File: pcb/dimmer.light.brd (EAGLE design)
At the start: 45.7 x 45.4 mm, 25 parts, among them IC1 NCP1117ST50T3G, SW1 RJ45SMD, T1 IRFR024NPBF, T2 BC847BSMD, U1 ATTINY2313

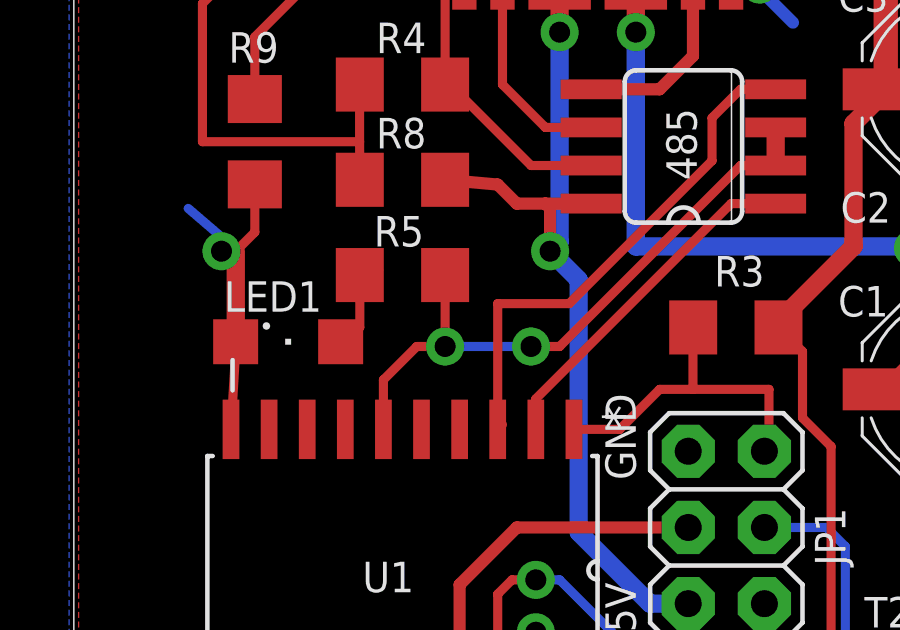
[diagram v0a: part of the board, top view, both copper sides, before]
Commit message: final version
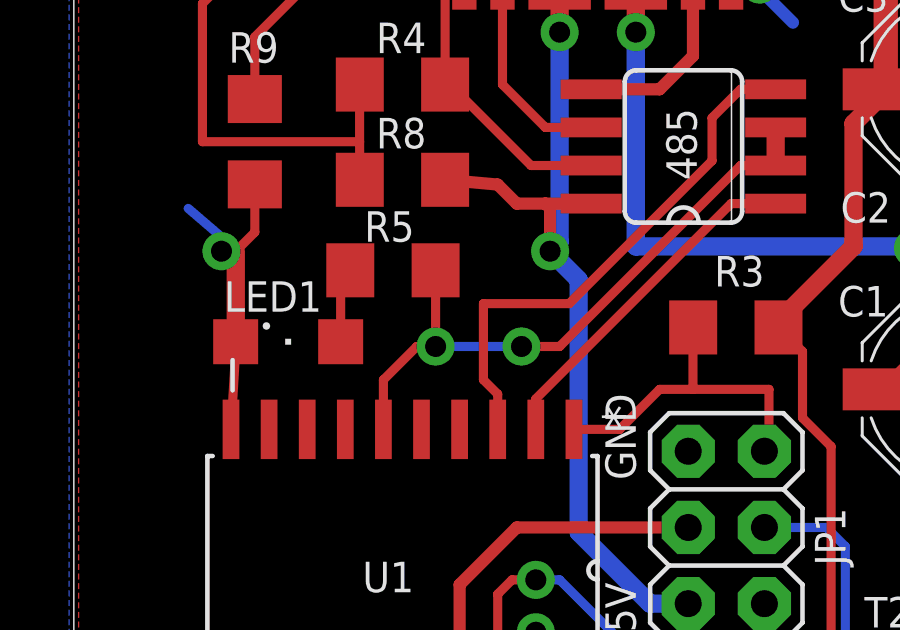
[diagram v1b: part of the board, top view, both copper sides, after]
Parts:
- R4: value 120 -> 220
- moved R5 0.35 mm to (12.9, 24.8)
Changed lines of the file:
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@@
 <attribute name="NAME" x="21.971" y="30.1625" size="1.016" layer="25" ratio="10" rot="R270"/>
 </element>
-<element name="R4" library="rcl" package="R1206" value="120" x="13.17625" y="30.95625" smashed="yes" rot="R180">
+<element name="R4" library="rcl" package="R1206" value="220" x="13.17625" y="30.95625" smashed="yes" rot="R180">
 <attribute name="NAME" x="13.97" y="33.02" size="1.016" layer="25" rot="R180"/>
 <attribute name="VALUE" x="14.44625" y="33.49625" size="1.27" layer="27" rot="R180"/>
@@
 <attribute name="VALUE" x="7.86625" y="19.88375" size="1.27" layer="27"/>
 </element>
-<element name="R5" library="rcl" package="R1206" value="680" x="13.17625" y="24.60625" smashed="yes">
-<attribute name="NAME" x="12.22375" y="25.55875" size="1.016" layer="25"/>
-<attribute name="VALUE" x="11.90625" y="22.06625" size="1.27" layer="27"/>
+<element name="R5" library="rcl" package="R1206" value="680" x="12.85875" y="24.765" smashed="yes">
+<attribute name="NAME" x="11.90625" y="25.7175" size="1.016" layer="25"/>
+<attribute name="VALUE" x="11.58875" y="22.225" size="1.27" layer="27"/>
 </element>
 <element name="R8" library="rcl" package="R1206" value="10k" x="13.17625" y="27.78125" smashed="yes">
@@
 <contactref element="LED1" pad="A"/>
 <contactref element="R5" pad="1"/>
-<wire x1="12.3855" y1="24.76875" x2="11.75425" y2="24.60625" width="0.3048" layer="1"/>
-<wire x1="11.75425" y1="24.60625" x2="11.75425" y2="22.863" width="0.3048" layer="1"/>
-<wire x1="11.75425" y1="22.863" x2="11.11625" y2="22.38375" width="0.3048" layer="1"/>
+<wire x1="11.43675" y1="24.765" x2="11.11625" y2="24.765" width="0.3048" layer="1"/>
+<wire x1="11.11625" y1="24.765" x2="11.11625" y2="22.38375" width="0.3048" layer="1"/>
 </signal>
 <signal name="N$18">
 <contactref element="485" pad="4"/>
 <contactref element="U1" pad="3"/>
-<wire x1="16.51" y1="19.6215" x2="16.35125" y2="19.46275" width="0.3048" layer="1"/>
 <wire x1="23.495" y1="28.41625" x2="18.7325" y2="23.65375" width="0.3048" layer="1"/>
-<wire x1="18.7325" y1="23.65375" x2="16.35125" y2="23.65375" width="0.3048" layer="1"/>
-<wire x1="16.35125" y1="23.65375" x2="16.35125" y2="19.46275" width="0.3048" layer="1"/>
+<wire x1="18.7325" y1="23.65375" x2="15.875" y2="23.65375" width="0.3048" layer="1"/>
 <wire x1="23.495" y1="28.41625" x2="23.495" y2="29.845" width="0.3048" layer="1"/>
 <wire x1="23.495" y1="29.845" x2="24.4475" y2="30.7975" width="0.3048" layer="1"/>
 <wire x1="24.4475" y1="30.7975" x2="25.6159" y2="30.7975" width="0.3048" layer="1"/>
+<wire x1="15.875" y1="23.65375" x2="15.875" y2="21.11375" width="0.3048" layer="1"/>
+<wire x1="15.875" y1="21.11375" x2="16.35125" y2="20.6375" width="0.3048" layer="1"/>
+<wire x1="16.35125" y1="20.6375" x2="16.35125" y2="19.46275" width="0.3048" layer="1"/>
 </signal>
 <signal name="N$19">
@@
 <contactref element="U1" pad="6"/>
 <wire x1="24.4475" y1="28.2575" x2="25.6159" y2="28.2575" width="0.3048" layer="1"/>
-<via x="17.4625" y="22.225" extent="1-16" drill="0.7" diameter="1.27" shape="square"/>
-<wire x1="14.605" y1="22.225" x2="14.59825" y2="22.225" width="0.3048" layer="16"/>
+<via x="17.145" y="22.225" extent="1-16" drill="0.7" diameter="1.27" shape="square"/>
+<wire x1="14.605" y1="22.225" x2="14.28075" y2="22.225" width="0.3048" layer="16"/>
 <wire x1="12.54125" y1="19.46275" x2="12.54125" y2="21.11375" width="0.3048" layer="1"/>
 <wire x1="12.54125" y1="21.11375" x2="13.6525" y2="22.225" width="0.3048" layer="1"/>
-<wire x1="13.6525" y1="22.225" x2="14.59825" y2="22.225" width="0.3048" layer="1"/>
-<via x="14.59825" y="22.225" extent="1-16" drill="0.7" diameter="1.27" shape="square"/>
-<wire x1="14.59825" y1="22.225" x2="17.4625" y2="22.225" width="0.3048" layer="16"/>
-<wire x1="14.59825" y1="24.60625" x2="14.59825" y2="22.225" width="0.3048" layer="1"/>
-<wire x1="17.4625" y1="22.225" x2="18.415" y2="22.225" width="0.3048" layer="1"/>
+<wire x1="13.6525" y1="22.225" x2="14.28075" y2="22.225" width="0.3048" layer="1"/>
+<via x="14.28075" y="22.225" extent="1-16" drill="0.7" diameter="1.27" shape="square"/>
+<wire x1="14.28075" y1="22.225" x2="17.145" y2="22.225" width="0.3048" layer="16"/>
+<wire x1="14.28075" y1="24.765" x2="14.28075" y2="22.225" width="0.3048" layer="1"/>
+<wire x1="17.145" y1="22.225" x2="18.415" y2="22.225" width="0.3048" layer="1"/>
 <wire x1="18.415" y1="22.225" x2="24.4475" y2="28.2575" width="0.3048" layer="1"/>
 </signal>
